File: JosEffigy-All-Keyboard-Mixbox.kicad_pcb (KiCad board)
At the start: 2 copper layers, 173 x 117.5 mm, 33 parts, among them U1 RP2040

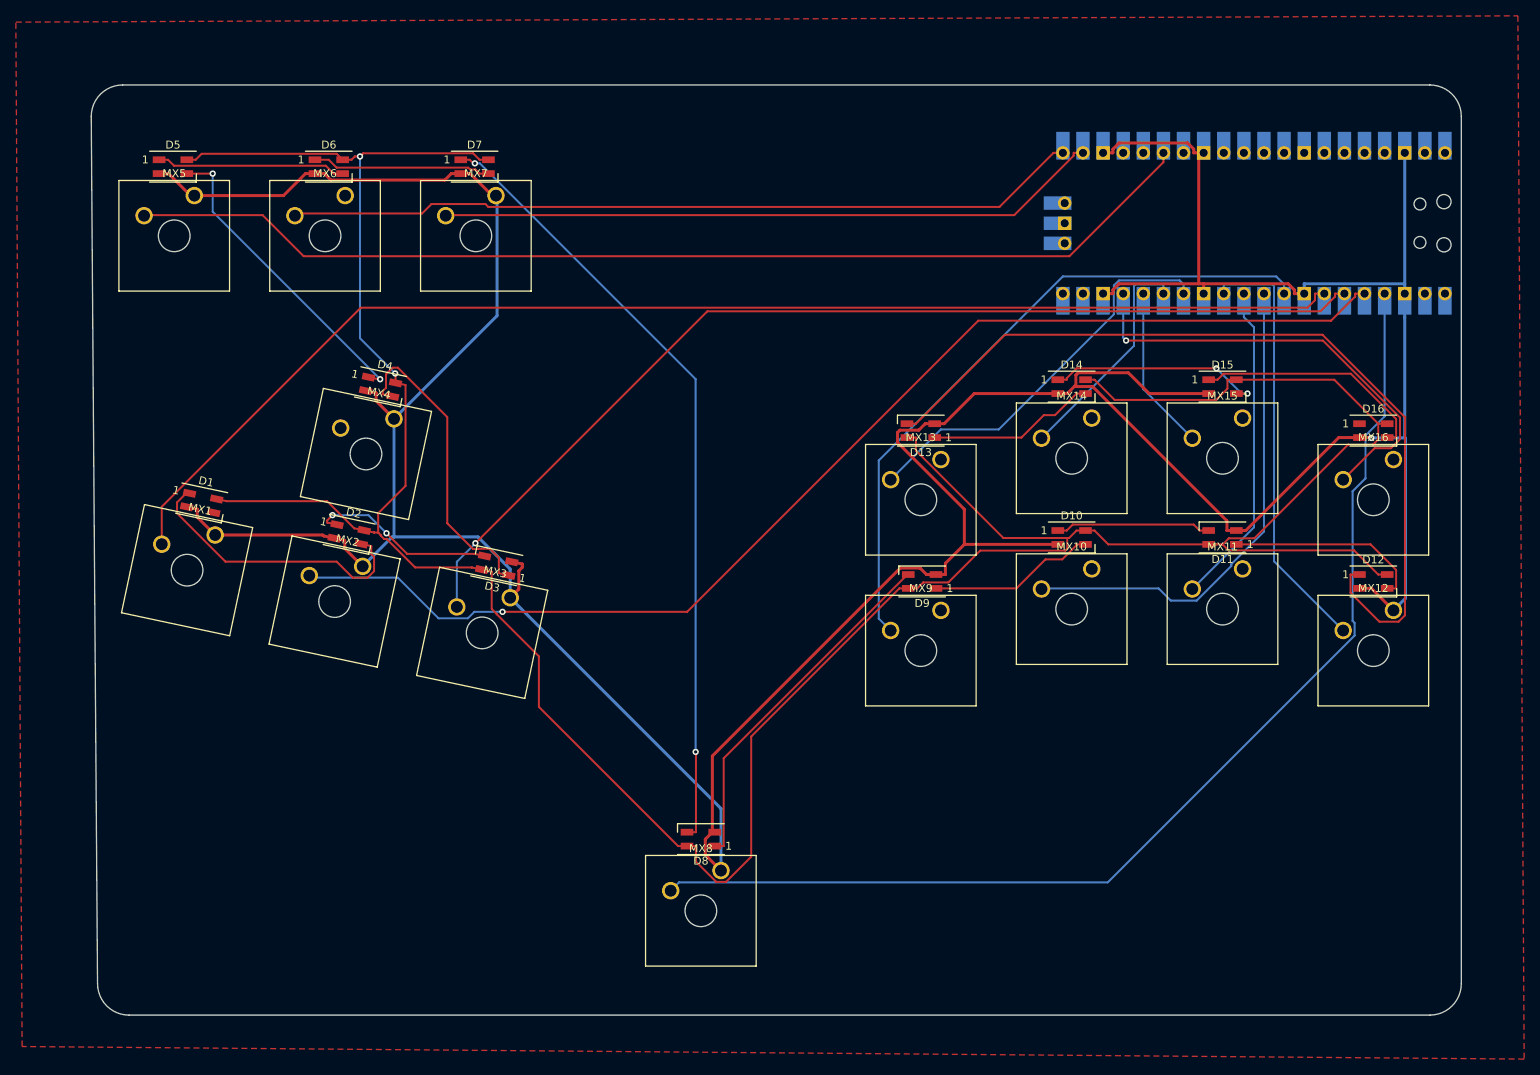
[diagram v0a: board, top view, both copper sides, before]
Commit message: Release 1.0
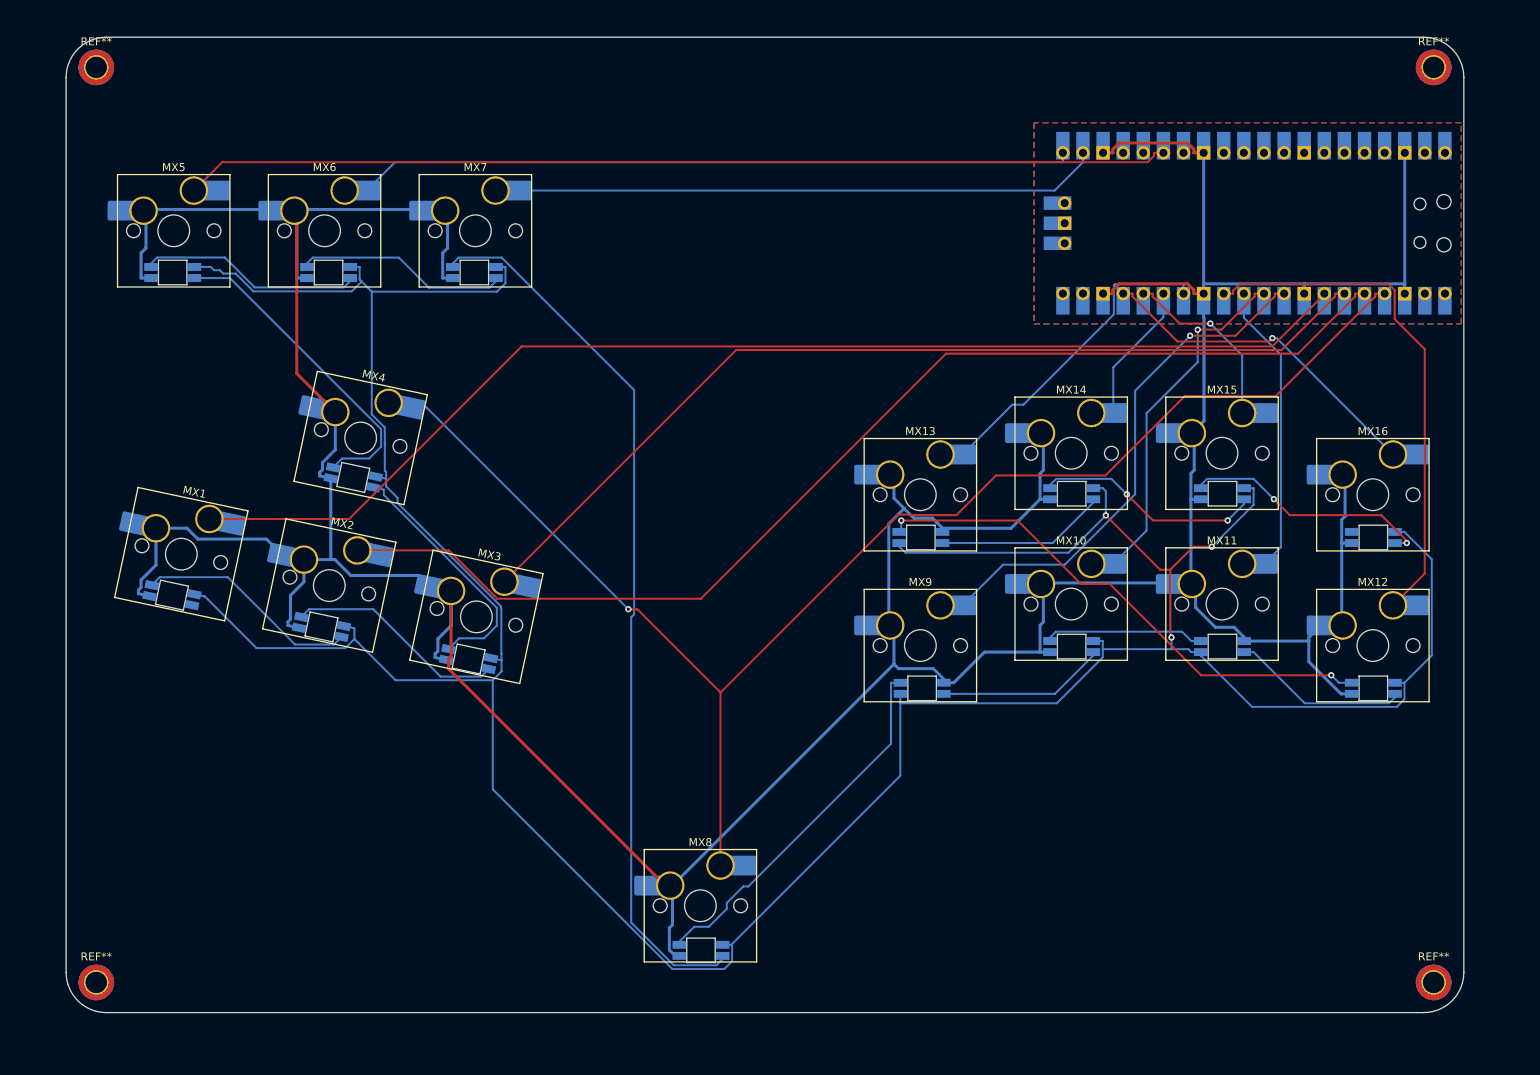
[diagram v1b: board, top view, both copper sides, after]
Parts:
- added REF**: MountingHole_2.7mm_M2.5_ISO7380_Pad_TopBottom, MountingHole:MountingHole_2.7mm_M2.5_ISO7380_Pad_TopBottom, F.Cu at (61.0, 156.2)
- added REF**: MountingHole_2.7mm_M2.5_ISO7380_Pad_TopBottom, MountingHole:MountingHole_2.7mm_M2.5_ISO7380_Pad_TopBottom, F.Cu at (229.9, 40.6)
- added REF**: MountingHole_2.7mm_M2.5_ISO7380_Pad_TopBottom, MountingHole:MountingHole_2.7mm_M2.5_ISO7380_Pad_TopBottom, F.Cu at (229.9, 156.2)
- added REF**: MountingHole_2.7mm_M2.5_ISO7380_Pad_TopBottom, MountingHole:MountingHole_2.7mm_M2.5_ISO7380_Pad_TopBottom, F.Cu at (61.0, 40.6)
- D1, D10, D11, D12, D13, D14, D15, D16, D2, D3, D4, D5, D6, D7, D8, D9: footprint LED_SMD:LED_SK6812MINI_PLCC4_3.5x3.5mm_P1.75mm -> kicad-footprints:YS-SK6812MINI-E; moved to B.Cu
- MX1, MX10, MX11, MX12, MX13, MX14, MX15, MX16, MX2, MX3, MX4, MX5, MX6, MX7, MX9: footprint Button_Switch_Keyboard:SW_Cherry_MX_1.00u_Plate -> PCM_Switch_Keyboard_Hotswap_Kailh:SW_Hotswap_Kailh_MX_Plated_1.00u
- MX8: footprint Button_Switch_Keyboard:SW_Cherry_MX_2.00u_Plate -> PCM_Switch_Keyboard_Hotswap_Kailh:SW_Hotswap_Kailh_MX_Plated_2.00u
- moved D8 14.1 mm to (137.3, 152.2)
- moved D10 13.8 mm to (184.2, 113.8), turned to 180 degrees
- moved D11 13.8 mm to (203.2, 113.8), turned to 0 degrees
- moved D14 13.5 mm to (184.2, 94.5), turned to 180 degrees
- moved D15 13.5 mm to (203.2, 94.5), turned to 180 degrees
- moved D13 13.5 mm to (165.1, 100.0), turned to 0 degrees
- moved D16 13.5 mm to (222.2, 100.0), turned to 180 degrees
- moved D12 13.5 mm to (222.2, 119.1), turned to 180 degrees
- moved D9 13.5 mm to (165.3, 119.1), turned to 0 degrees
- moved D5 13.4 mm to (70.6, 66.5), turned to 180 degrees
- moved D6 13.4 mm to (90.3, 66.5), turned to 180 degrees
- moved D7 13.4 mm to (108.7, 66.5), turned to 180 degrees
- moved D3 12.3 mm to (108.0, 115.4)
- moved D1 12.2 mm to (70.5, 107.3), turned to 168 degrees
- moved D2 12.2 mm to (89.4, 111.3), turned to 168 degrees
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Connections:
- MX10 pad 1: unconnected-(MX10-COL-Pad1) -> GND
- MX11 pad 1: unconnected-(MX11-COL-Pad1) -> GND
- MX13 pad 1: unconnected-(MX13-COL-Pad1) -> GND
- MX14 pad 1: unconnected-(MX14-COL-Pad1) -> GND
- MX15 pad 1: unconnected-(MX15-COL-Pad1) -> GND
- MX16 pad 1: unconnected-(MX16-COL-Pad1) -> GND
- MX4 pad 2: unconnected-(MX4-ROW-Pad2) -> UP
- MX6 pad 1: unconnected-(MX6-COL-Pad1) -> GND
- MX9 pad 1: unconnected-(MX9-COL-Pad1) -> GND
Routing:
- net GND: track 530.0 -> 606.9 mm, vias 1 -> 0
- net Net-(D12-DOUT): track 109.0 -> 66.9 mm, vias 0 -> 2
- net UP: track 144.7 -> 186.7 mm, vias 0 -> 1
- net VCC: track 393.5 -> 421.9 mm, vias 2 -> 3
- net 1K: track 84.5 -> 67.6 mm, vias 0 -> 1
- net 2K: track 62.6 -> 47.2 mm, vias 0 -> 1
- net 4K: track 54.7 -> 68.4 mm
- net Net-(D7-DOUT): track 99.5 -> 112.5 mm, vias 2 -> 0
- net 4P: track 56.7 -> 45.8 mm
- net HOME: track 137.0 -> 127.4 mm
- net 2P: track 29.1 -> 20.5 mm
- net Net-(D1-DOUT): track 36.6 -> 28.3 mm
- net 1P: track 50.9 -> 42.9 mm
- net Net-(D3-DOUT): track 39.7 -> 31.8 mm
- net RIGHT: track 132.0 -> 124.3 mm, vias 1 -> 0
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- added copper zone on B.Cu, net GND
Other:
- board size 173 x 117.5 mm -> 176.5 x 123.2 mm
